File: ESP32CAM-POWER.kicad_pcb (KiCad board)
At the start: 2 copper layers, 80 x 80 mm, 53 parts, among them J1 Screw_Terminal_01x02, J2 Conn_01x06_Male, SW1 TS-1187A-B-A-B, U2 ESP32-CAM, U3 XL1509-5.0E1

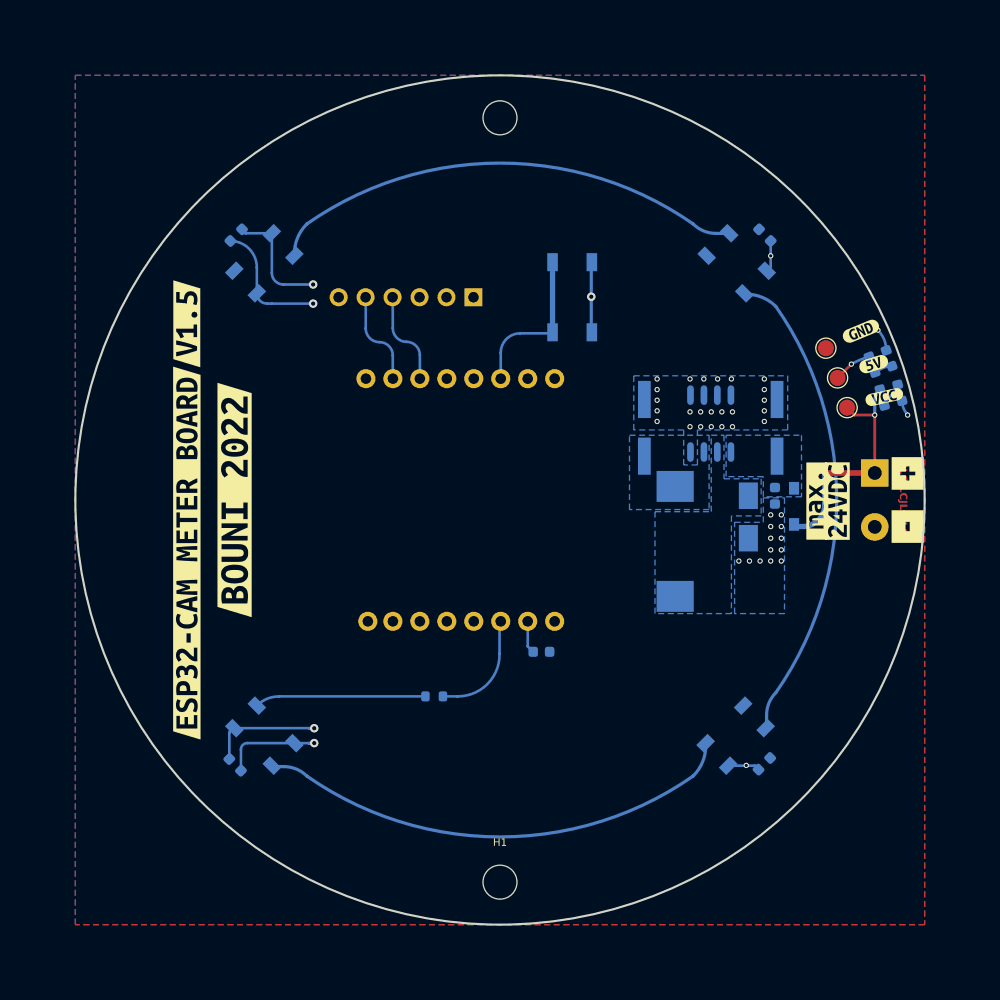
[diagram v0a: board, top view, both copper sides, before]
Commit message: Ooctober 2024 Update
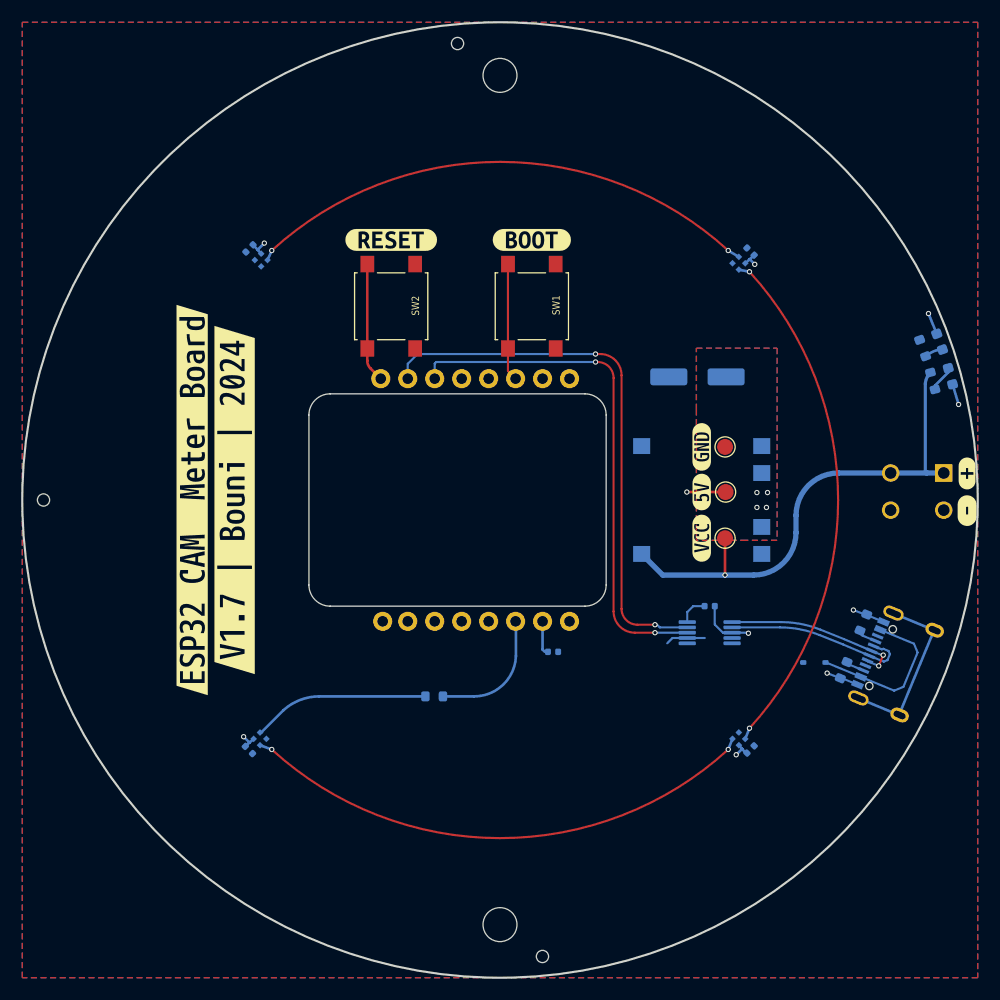
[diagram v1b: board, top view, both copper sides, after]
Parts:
- removed C9: 100uF/35V, LCSC:CAP-SMD_BD6.3-L6.6-W6.6-LS7.6-FD
- removed D4: SS54, Diode_SMD:D_SMA
- removed L1: 68uH / 2A, LCSC:IND-SMD_L11.5-W10.0_SMMS1040
- removed U3: XL1509-5.0E1, LCSC:SOP-8_L4.9-W3.9-P1.27-LS6.0-BL
- removed kibuzzard-611BC015: G***, kibuzzard-611BC015
- removed kibuzzard-61C9B205: G***, kibuzzard-61C9B205
- removed kibuzzard-61CABD37: G***, kibuzzard-61CABD37
- removed kibuzzard-61CABD72: G***, kibuzzard-61CABD72
- removed kibuzzard-62976FF9: G***, kibuzzard-62976FF9
- removed kibuzzard-62977004: G***, kibuzzard-62977004
- removed kibuzzard-62977011: G***, kibuzzard-62977011
- removed kibuzzard-62989351: G***, kibuzzard-62989351
- removed kibuzzard-6298938A: G***, kibuzzard-6298938A
- removed kibuzzard-62B5A597: G***, kibuzzard-62B5A597
- removed kibuzzard-62B5A6D7: G***, kibuzzard-62B5A6D7
- removed kibuzzard-62B5A6E6: G***, kibuzzard-62B5A6E6
- removed kibuzzard-62B5A6F5: G***, kibuzzard-62B5A6F5
- removed kibuzzard-62B5A702: G***, kibuzzard-62B5A702
- removed kibuzzard-62B5A718: G***, kibuzzard-62B5A718
- removed kibuzzard-62B5A722: G***, kibuzzard-62B5A722
- removed kibuzzard-62B5A742: G***, kibuzzard-62B5A742
- removed kibuzzard-62B5A752: G***, kibuzzard-62B5A752
- removed kibuzzard-62B5BECB: G***, kibuzzard-62B5BECB
- removed kibuzzard-62B5C3E7: G***, kibuzzard-62B5C3E7
- removed kibuzzard-62B5C3FB: G***, kibuzzard-62B5C3FB
- removed kibuzzard-62B5C445: G***, kibuzzard-62B5C445
- removed kibuzzard-62B5C484: G***, kibuzzard-62B5C484
- added PS1: TSR_1-2450SM, TRACO-TSR1:TSR124120SM, B.Cu at (169.0, 80.0)
- added R4: 5K1, Resistor_SMD:R_0603_1608Metric, B.Cu at (184.2, 91.5)
- added R5: 5K1, Resistor_SMD:R_0603_1608Metric, B.Cu at (182.4, 96.0)
- added SW2: SW_Omron_B3S, Button_Switch_SMD:SW_SPST_B3S-1000, F.Cu at (139.8, 61.8)
- added TH: ToolingHole, JLCPCB:ToolingHole, F.Cu at (146.0, 37.0)
- added TH: ToolingHole, JLCPCB:ToolingHole, F.Cu at (107.0, 80.0)
- added TH: ToolingHole, JLCPCB:ToolingHole, F.Cu at (154.0, 123.0)
- added U1: CH340X, Package_SO:MSOP-10_3x3mm_P0.5mm, B.Cu at (169.8, 92.5)
- added kibuzzard-66C75903: G***, kibuzzard-66C75903, F.Cu at (153.0, 55.5)
- added kibuzzard-66C7590B: G***, kibuzzard-66C7590B, F.Cu at (139.8, 55.5)
- added kibuzzard-66C81FD1: G***, kibuzzard-66C81FD1, F.Cu at (121.0, 80.0)
- added kibuzzard-66C81FE3: G***, kibuzzard-66C81FE3, F.Cu at (125.0, 80.0)
- added kibuzzard-66C82011: G***, kibuzzard-66C82011, F.Cu at (194.0, 77.5)
- added kibuzzard-66C8202D: G***, kibuzzard-66C8202D, F.Cu at (194.0, 81.0)
- added kibuzzard-66CDCC8A: G***, kibuzzard-66CDCC8A, F.Cu at (169.0, 83.6)
- added kibuzzard-66CDCC90: G***, kibuzzard-66CDCC90, F.Cu at (169.0, 79.2)
- added kibuzzard-66CDCC95: G***, kibuzzard-66CDCC95, F.Cu at (169.0, 75.0)
- C1, C2, C3, C4, C5: footprint Capacitor_SMD:C_0603_1608Metric -> Capacitor_SMD:C_0402_1005Metric
- C6: value 100uF/35V -> 0.1uF; footprint LCSC:CAP-SMD_BD6.3-L6.6-W6.6-LS7.6-FD -> Capacitor_SMD:C_0402_1005Metric
- C7: value 0.1uF -> 100uF; footprint Capacitor_SMD:C_0603_1608Metric -> Capacitor_SMD:CP_Elec_6.3x5.8
- D1: value LED_Y -> LED_B
- D3: value D_Schottky -> 1N5819WS; footprint LCSC:SOD-123_L2.7-W1.6-LS3.7-RD-1 -> Diode_SMD:D_SOD-323
- J1: footprint TerminalBlock_Phoenix:TerminalBlock_Phoenix_MKDS-1,5-2-5.08_1x02_P5.08mm_Horizontal -> SPTAF1:1861933
- J2: value Conn_01x06_Male -> USB_C_Receptacle_USB2.0_16P; footprint Connector_PinHeader_2.54mm:PinHeader_1x06_P2.54mm_Vertical -> LCSC:USB-C-SMD_TYPE-C-6PIN-2MD-073
- LED1, LED2, LED3, LED4: value XL-5050RGBC-WS2812B -> XL-1010RGBC-WS2812B; footprint LCSC:LED-SMD_4P-L5.0-W5.0-BL_XL-5050RGBC -> LCSC:LED-SMD_4P-L1.0-W1.0-TL_XL-1010RGBC-WS2812B
- SW1: value TS-1187A-B-A-B -> SW_Omron_B3S; footprint LCSC:SW-SMD_4P-L5.1-W5.1-P3.70-LS6.5-TL-2 -> Button_Switch_SMD:SW_SPST_B3S-1000; moved to F.Cu
- moved J2 52.5 mm to (187.1, 95.3), turned to -112.5 degrees
- moved C6 17.9 mm to (169.8, 90.0), turned to 180 degrees
- moved TP3 16.8 mm to (171.2, 83.6)
- moved TP2 15.1 mm to (171.2, 79.2)
- moved D3 14.8 mm to (179.6, 95.3), turned to 0 degrees
- moved C7 13.4 mm to (168.6, 68.4), turned to 0 degrees
- moved TP1 13.3 mm to (171.2, 75.0)
- moved J1 6.50 mm to (191.8, 77.5)
- moved D1 5.01 mm to (192.4, 68.3)
- moved D2 5.01 mm to (191.4, 65.1)
- moved R2 5.01 mm to (189.8, 65.7)
- moved R1 5.01 mm to (190.8, 68.8)
- moved H1 4.00 mm to (150.0, 120.0)
- moved H2 4.00 mm to (150.0, 40.0)
- moved SW1 3.89 mm to (153.0, 61.8), turned to -90 degrees
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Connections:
- C6 pad 1: +5V -> GND
- C6 pad 2: GND -> Net-(U1-V3)
- C7 pad 1: /VIN -> +5V
- D3 pad 1: /VIN -> +5V
- D3 pad 2: VCC -> Net-(D3-A)
- LED1 pad 1: +5V -> D1
- LED1 pad 2: Net-(LED1-DO) -> +5V
- LED1 pad 3: Net-(LED1-DI) -> GND
- LED1 pad 4: GND -> Net-(LED1-DIN)
- LED2 pad 1: +5V -> D2
- LED2 pad 2: Net-(LED2-DO) -> +5V
- LED2 pad 3: Net-(LED1-DO) -> GND
- LED2 pad 4: GND -> D1
- LED3 pad 1: +5V -> D3
- LED3 pad 2: Net-(LED3-DO) -> +5V
- LED3 pad 3: Net-(LED2-DO) -> GND
- LED3 pad 4: GND -> D2
- LED4 pad 1: +5V -> unconnected-(LED4-DOUT-Pad1)
- LED4 pad 2: unconnected-(LED4-DO) -> +5V
- LED4 pad 3: Net-(LED3-DO) -> GND
- LED4 pad 4: GND -> D3
- R3 pad 2: Net-(LED1-DI) -> Net-(LED1-DIN)
- SW1 pad 2: GND -> BOOT
- U2 pad 14: RX -> TXD
- U2 pad 15: TX -> RXD
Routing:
- net RXD: track 0.00 -> 52.1 mm, vias 0 -> 2
- net TXD: track 0.00 -> 49.1 mm, vias 0 -> 2
- net Net-(LED1-DO): track 45.3 -> 0.00 mm
- net Net-(LED3-DO): track 45.3 -> 0.00 mm
- net Net-(LED2-DO): track 44.9 -> 0.00 mm
- net VCC: track 22.4 -> 48.3 mm, vias 2 -> 1
- net /D-: track 0.00 -> 17.7 mm
- net +5V: track 24.9 -> 7.41 mm, vias 3 -> 1
- net /D+: track 0.00 -> 17.1 mm, vias 0 -> 2
- net unconnected-(J2-SHIELD-PadS1): track 0.00 -> 17.1 mm
- net Net-(LED1-DIN): track 0.00 -> 16.7 mm
- net Net-(LED1-DI): track 16.1 -> 0.00 mm
- net Net-(D3-A): track 0.00 -> 15.8 mm
- net GND: track 41.3 -> 25.9 mm, vias 44 -> 13
- net RESET: track 0.00 -> 11.3 mm
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- removed copper zone on B.Cu, net /OUT
- removed copper zone on B.Cu, net /VIN
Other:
- board size 80 x 80 mm -> 90 x 90 mm
